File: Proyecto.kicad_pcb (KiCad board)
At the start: 2 copper layers, 149.9 x 100.1 mm, 40 parts, among them J10 PORTC, J11 PORTE, J12 Pickit 3, J2 Alimentacion, J3 LCD, J4 Teclado, J5 hc-06, J6 PORTA, J7 Vusb, J8 PORTB, J9 PORTD, SW1 Power/Acticidad/Cuidado, U1 NRF24L01_Breakout, U2 Fuente de 9-5v, U3 PIC18F4550-IP, U4 Fuente de 3.3v

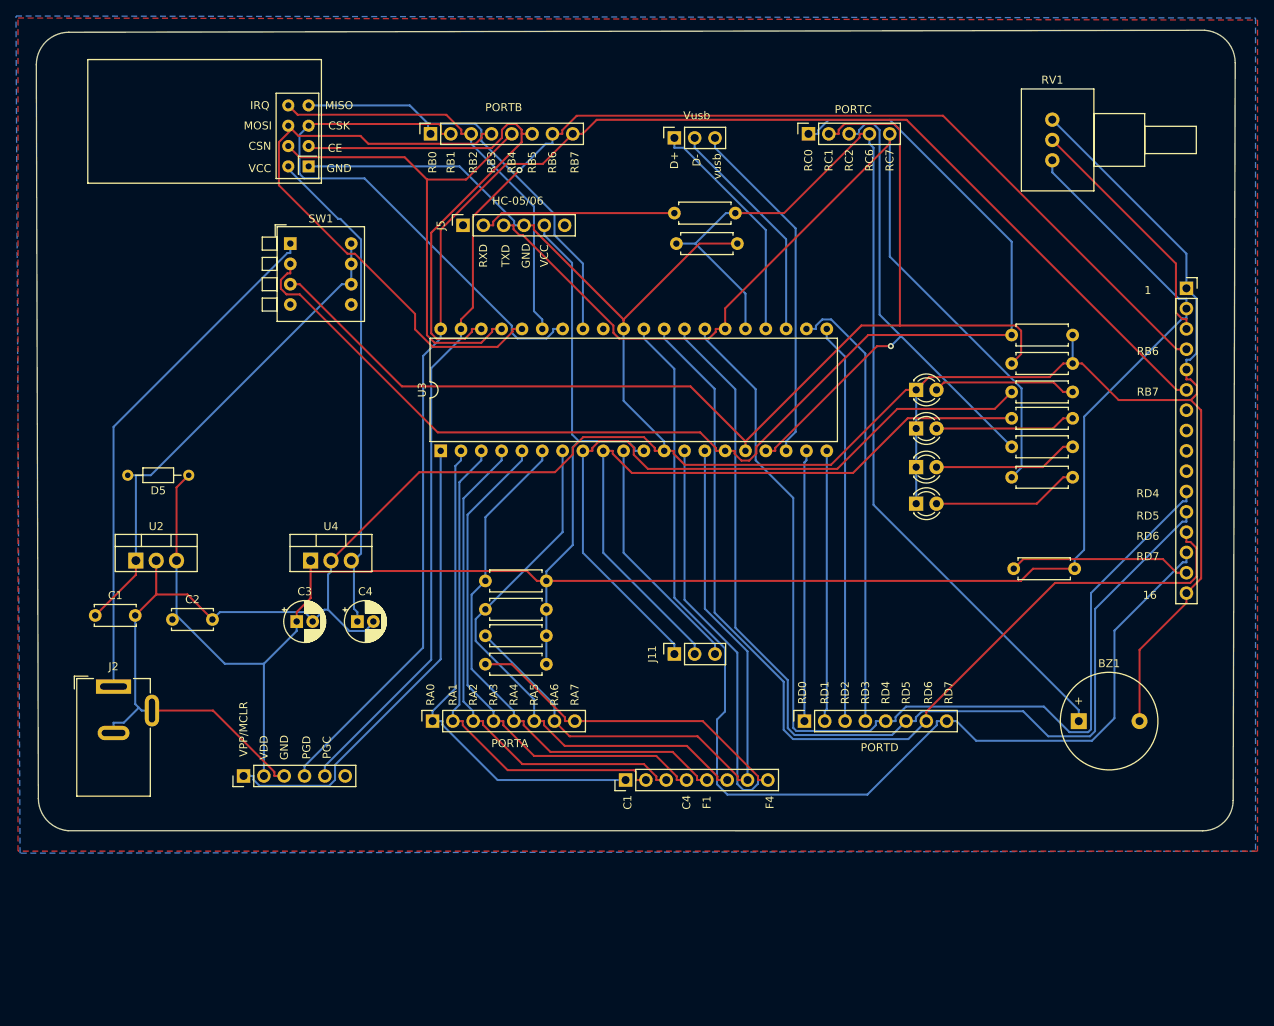
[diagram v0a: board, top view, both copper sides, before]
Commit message: version 1.5
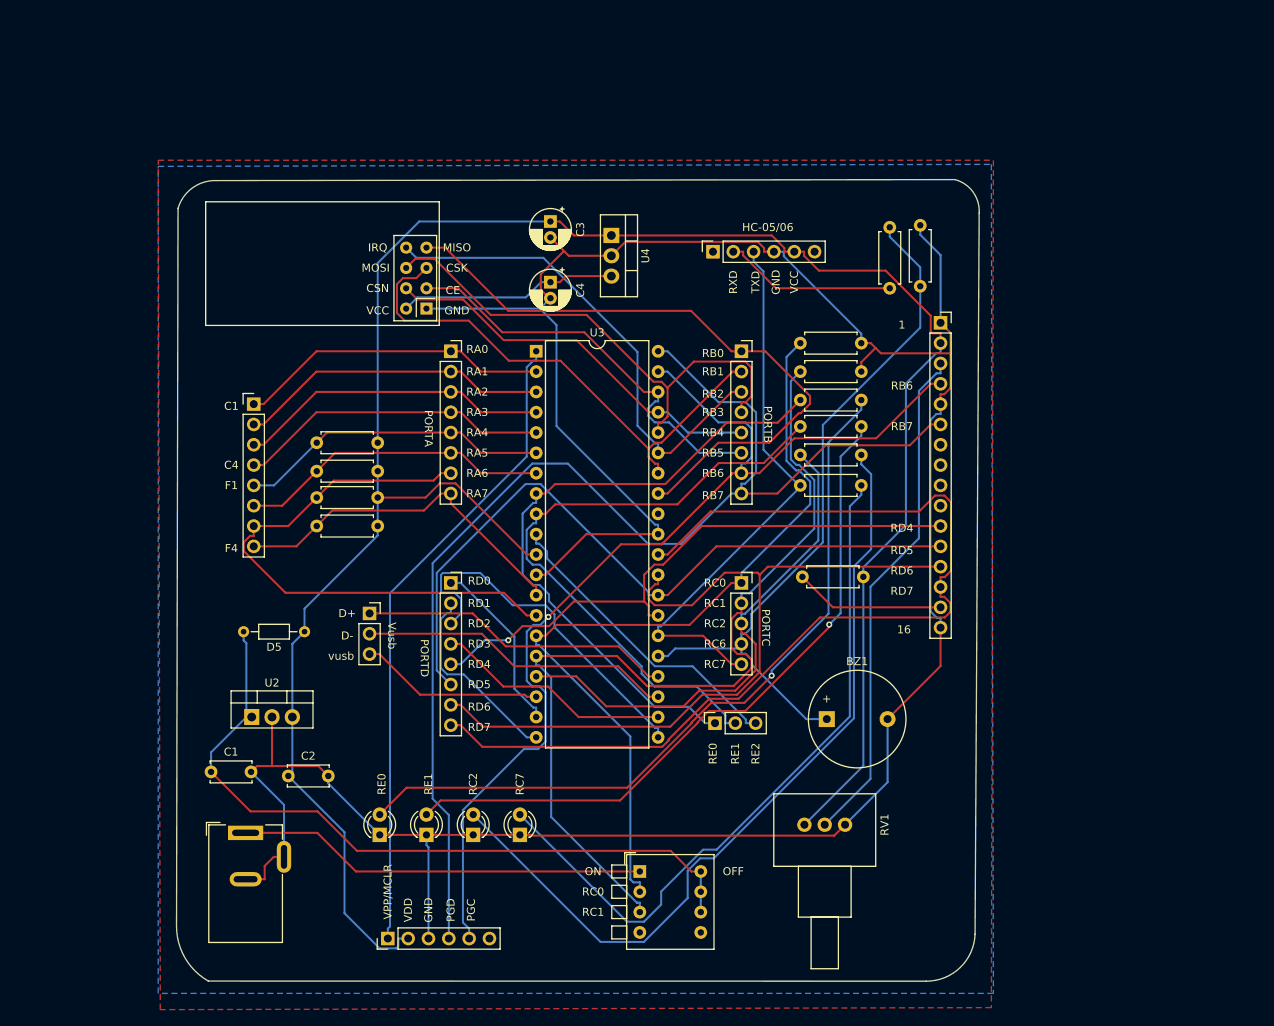
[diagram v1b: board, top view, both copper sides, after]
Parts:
- moved SW1 89.8 mm to (149.1, 142.5)
- moved RV1 88.7 mm to (169.7, 136.7), turned to 270 degrees
- moved D1 87.1 mm to (116.6, 137.9), turned to 90 degrees
- moved D2 79.5 mm to (122.4, 137.9), turned to 90 degrees
- moved D3 72.0 mm to (128.3, 137.9), turned to 90 degrees
- moved J7 70.6 mm to (115.3, 110.2), turned to 0 degrees
- moved J4 66.1 mm to (100.8, 84.1), turned to 0 degrees
- moved D4 64.6 mm to (134.1, 137.9), turned to 90 degrees
- moved C3 59.2 mm to (137.9, 61.2), turned to 270 degrees
- moved J10 56.8 mm to (161.8, 106.4), turned to 0 degrees
- moved U4 55.4 mm to (145.5, 63.0), turned to 270 degrees
- moved C4 48.8 mm to (137.9, 68.8), turned to 270 degrees
- moved J9 47.5 mm to (125.5, 106.4), turned to 0 degrees
- moved J8 47.4 mm to (161.8, 77.5), turned to 0 degrees
- moved J6 46.3 mm to (125.5, 77.5), turned to 0 degrees
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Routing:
- net Net-(D3-Pad2): track 18.1 -> 102.1 mm
- net Net-(D1-Pad2): track 17.9 -> 95.3 mm, vias 0 -> 1
- net Net-(D4-Pad2): track 18.4 -> 87.8 mm
- net Net-(D2-Pad2): track 17.5 -> 86.8 mm, vias 0 -> 1
- net GND: track 398.9 -> 339.6 mm
- net /RD4: track 130.1 -> 73.5 mm, vias 0 -> 1
- net /RB6: track 185.1 -> 131.2 mm
- net /RC0: track 155.8 -> 102.1 mm
- net /RC7: track 118.3 -> 69.9 mm
- net /RA7: track 91.1 -> 44.7 mm
- net /RD5: track 129.5 -> 90.8 mm
- net /RC6: track 127.6 -> 89.6 mm
- net /RB7: track 188.2 -> 153.3 mm
- net /V3: track 61.7 -> 27.3 mm
- net /VEE: track 30.9 -> 64.0 mm
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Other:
- board size 149.9 x 100.1 mm -> 100.3 x 100.2 mm
- board text added: "OFF"
- board text added: "ON"
- board text added: "RE0"
- board text added: "RE1"
- board text added: "RE2"
